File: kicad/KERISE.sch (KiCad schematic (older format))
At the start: 4 parts, among them SW1 SW_Push, U1 ESP32-PICO-D4

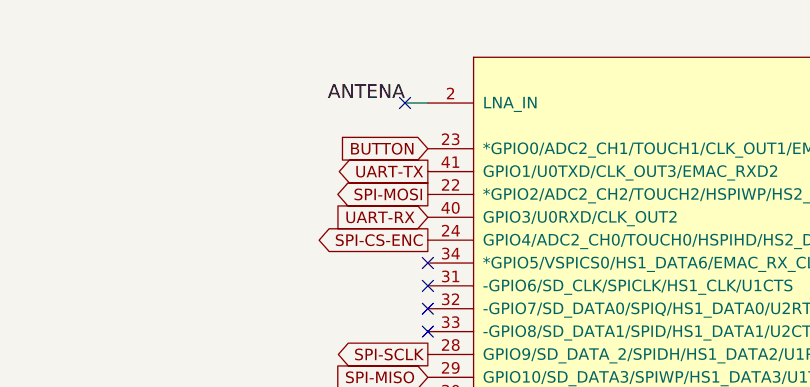
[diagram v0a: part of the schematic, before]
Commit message: 電源ラインを配線
あとは自動配線
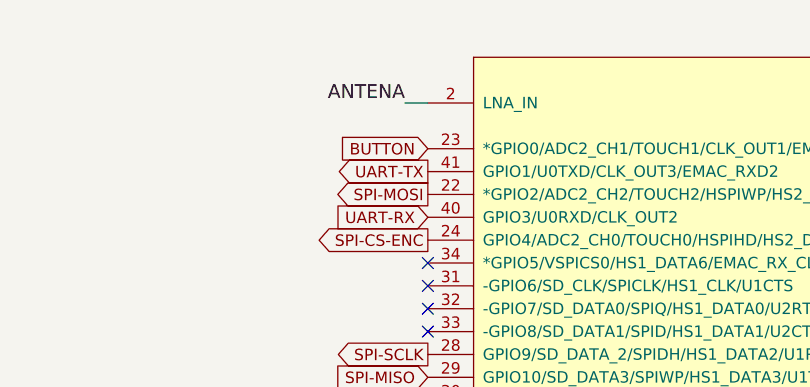
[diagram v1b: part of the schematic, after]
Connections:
- no-connect marks 14 -> 13
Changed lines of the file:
@@
 Connection ~ 9800 2100
 NoConn ~ 5600 1700
-NoConn ~ 5500 1000
 $EndSCHEMATC

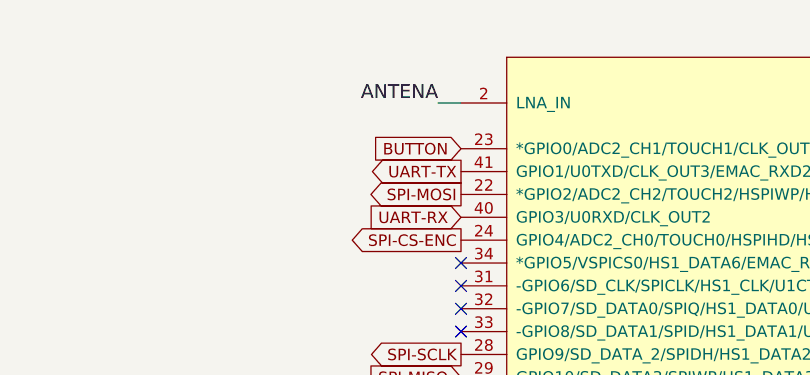
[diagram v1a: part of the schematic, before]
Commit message: 7本残して自動配線終了
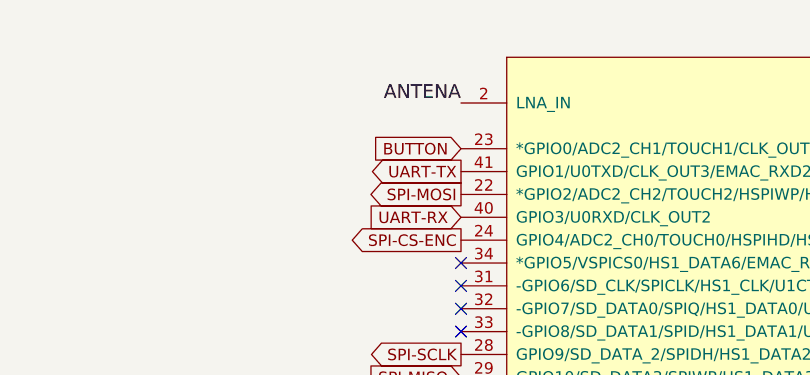
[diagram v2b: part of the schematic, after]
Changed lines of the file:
@@
 Text GLabel 5600 3400 0    50   Output ~ 0
 I2C-SCL
-Text Label 5500 1000 2    60   ~ 0
+Text Label 5600 1000 2    60   ~ 0
 ANTENA
-Wire Wire Line
-	5600 1000 5500 1000
 $Comp
 L ESP32-PICO-D4 U1
